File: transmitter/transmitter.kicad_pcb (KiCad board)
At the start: 2 copper layers, 8 parts, among them J1 Conn_01x05, J2 Conn_01x05, U1 NRF24L01_Breakout, U2 AMS1117-3.3

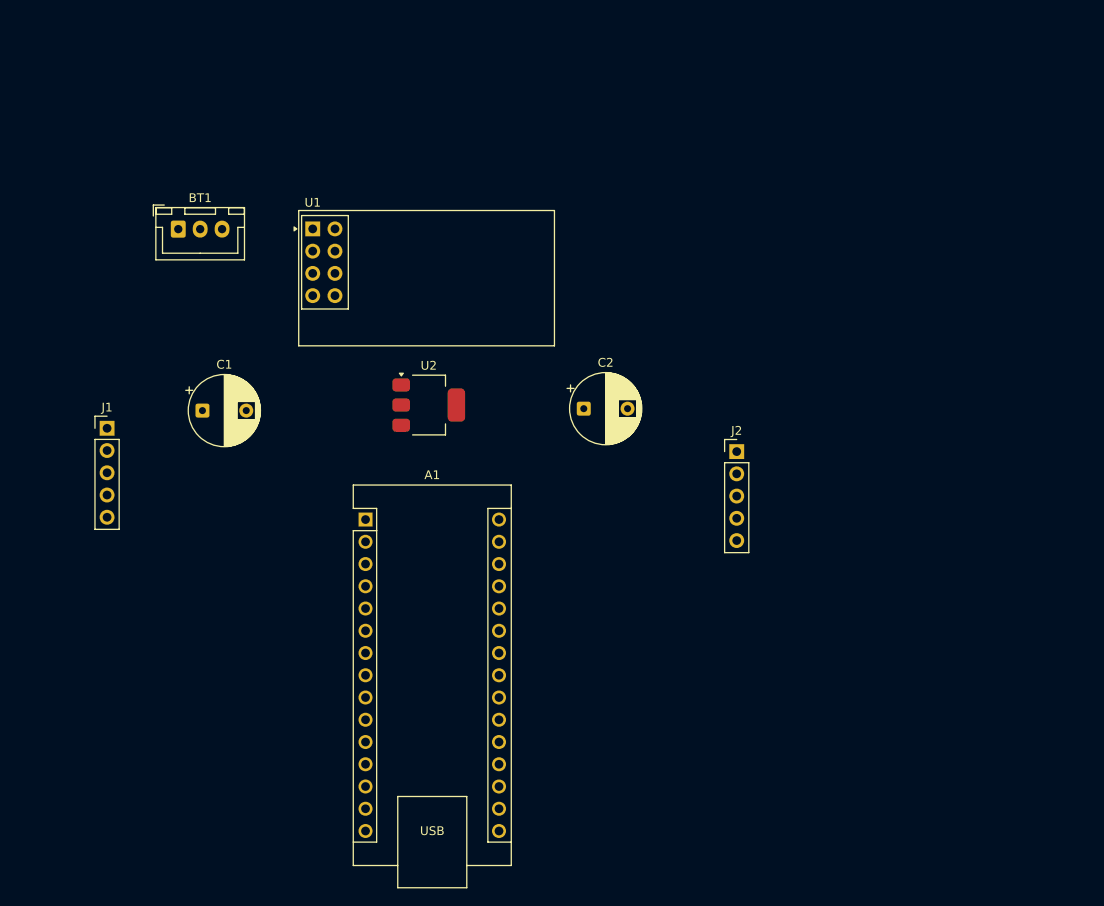
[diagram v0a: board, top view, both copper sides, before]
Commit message: Completed transmitter PCB and rough BOM, updated journal
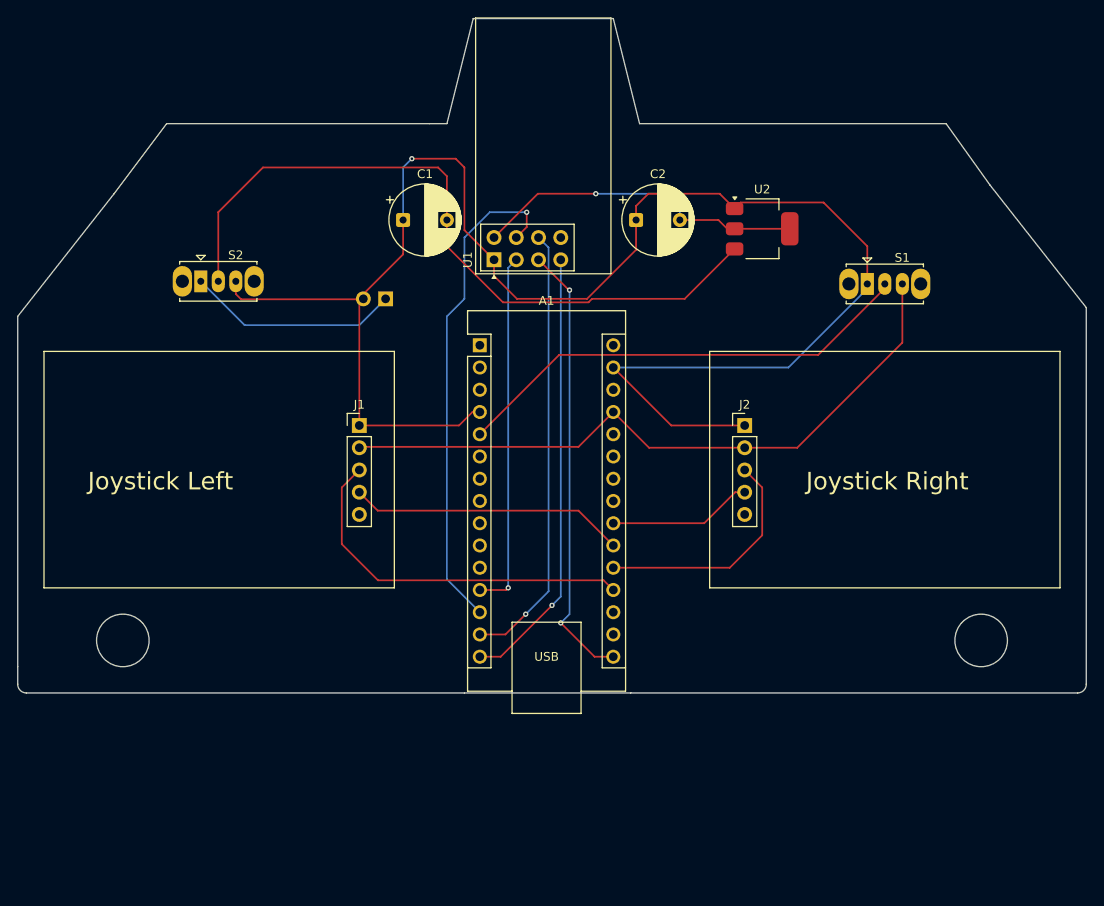
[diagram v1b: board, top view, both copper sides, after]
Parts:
- added S1: FlashLightToggle, Button_Switch_THT:SW_Slide_SPDT_Straight_CK_OS102011MS2Q, F.Cu at (210.0, 69.3)
- added S2: OnOff, Button_Switch_THT:SW_Slide_SPDT_Straight_CK_OS102011MS2Q, F.Cu at (133.9, 69.0)
- BT1: footprint Connector_JST:JST_XH_B3B-XH-A_1x03_P2.50mm_Vertical -> Connector_PinHeader_2.54mm:PinHeader_1x02_P2.54mm_Vertical; moved to B.Cu
- moved U2 43.1 mm to (198.0, 63.0)
- moved C1 31.6 mm to (157.0, 62.0)
- moved J1 28.8 mm to (152.0, 85.5)
- moved BT1 25.0 mm to (155.0, 71.0), turned to 90 degrees
- moved A1 23.8 mm to (165.8, 76.3)
- moved C2 22.4 mm to (183.6, 62.0)
- moved U1 21.0 mm to (167.4, 66.5), turned to 90 degrees
- moved J2 3.12 mm to (196.0, 85.5)
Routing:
- net GND: track 0.00 -> 193.8 mm, vias 0 -> 1
- net Net-(U2-VI): track 0.00 -> 82.6 mm
- net +5V: track 0.00 -> 77.1 mm
- net Net-(A1-D10): track 0.00 -> 56.9 mm, vias 0 -> 1
- net Net-(A1-D2): track 0.00 -> 53.6 mm
- net Net-(A1-SCK): track 0.00 -> 51.0 mm, vias 0 -> 2
- net Net-(A1-MOSI): track 0.00 -> 50.8 mm, vias 0 -> 1
- net Net-(A1-MISO): track 0.00 -> 50.5 mm, vias 0 -> 1
- net X1: track 0.00 -> 42.5 mm
- net Net-(A1-D9): track 0.00 -> 41.2 mm, vias 0 -> 1
- net +3.3V: track 0.00 -> 38.3 mm, vias 0 -> 1
- net Y1: track 0.00 -> 31.5 mm
- net X2: track 0.00 -> 26.8 mm
- net Net-(BT1-+): track 0.00 -> 24.4 mm
- net Y2: track 0.00 -> 16.5 mm
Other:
- board outline added: 122 x 77 mm
- board text added: "Joystick Left"
- board text added: "Joystick Right"
